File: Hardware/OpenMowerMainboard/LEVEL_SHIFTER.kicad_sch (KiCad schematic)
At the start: 3 parts, among them Q16 BSS138

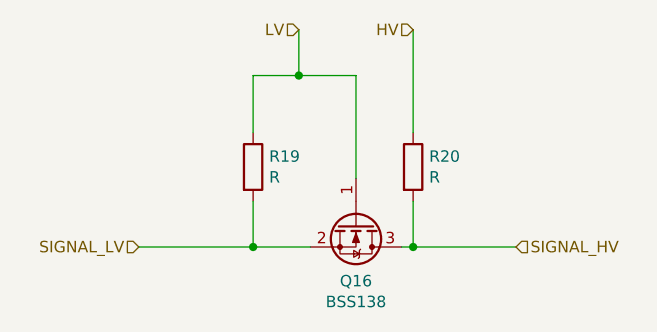
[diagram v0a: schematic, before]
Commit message: minor changes
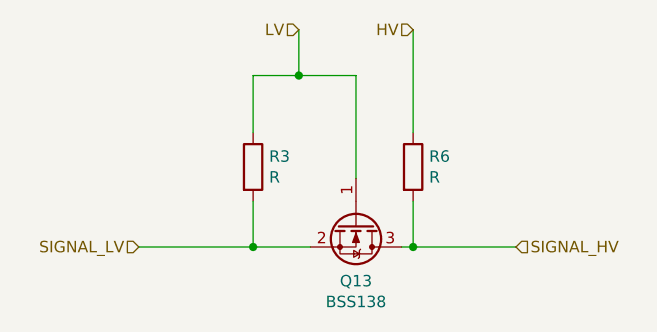
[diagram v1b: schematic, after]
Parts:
- renumbered Q16 to Q13, R19 to R3, R20 to R6
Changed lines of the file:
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@@
   (symbol (lib_id "Transistor_FET:BSS138") (at 114.3 76.2 270)
     (in_bom yes) (on_board yes)
-    (property "Reference" "Q16" (id 0) (at 114.3 82.5246 90))
+    (property "Reference" "Q13" (id 0) (at 114.3 82.5246 90))
     (property "Value" "BSS138" (id 1) (at 114.3 84.836 90))
     (property "Footprint" "Package_TO_SOT_SMD:SOT-23" (id 2) (at 112.395 81.28 0)
@@
   (symbol (lib_id "Device:R") (at 102.87 69.85 0)
     (in_bom yes) (on_board yes)
-    (property "Reference" "R19" (id 0) (at 104.648 68.6816 0)
+    (property "Reference" "R3" (id 0) (at 104.648 68.6816 0)
       (effects (font (size 1.27 1.27)) (justify left))
     )
@@
   (symbol (lib_id "Device:R") (at 120.65 69.85 0)
     (in_bom yes) (on_board yes)
-    (property "Reference" "R20" (id 0) (at 122.428 68.6816 0)
+    (property "Reference" "R6" (id 0) (at 122.428 68.6816 0)
       (effects (font (size 1.27 1.27)) (justify left))
     )

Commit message: minor changes
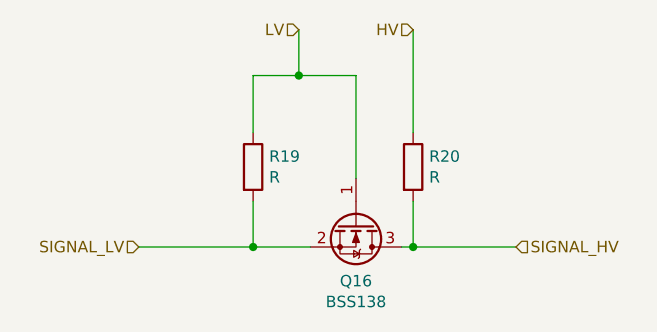
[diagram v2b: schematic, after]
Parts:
- renumbered Q13 to Q16, R3 to R19, R6 to R20
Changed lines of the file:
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@@
   (symbol (lib_id "Transistor_FET:BSS138") (at 114.3 76.2 270)
     (in_bom yes) (on_board yes)
-    (property "Reference" "Q13" (id 0) (at 114.3 82.5246 90))
+    (property "Reference" "Q16" (id 0) (at 114.3 82.5246 90))
     (property "Value" "BSS138" (id 1) (at 114.3 84.836 90))
     (property "Footprint" "Package_TO_SOT_SMD:SOT-23" (id 2) (at 112.395 81.28 0)
@@
   (symbol (lib_id "Device:R") (at 102.87 69.85 0)
     (in_bom yes) (on_board yes)
-    (property "Reference" "R3" (id 0) (at 104.648 68.6816 0)
+    (property "Reference" "R19" (id 0) (at 104.648 68.6816 0)
       (effects (font (size 1.27 1.27)) (justify left))
     )
@@
   (symbol (lib_id "Device:R") (at 120.65 69.85 0)
     (in_bom yes) (on_board yes)
-    (property "Reference" "R6" (id 0) (at 122.428 68.6816 0)
+    (property "Reference" "R20" (id 0) (at 122.428 68.6816 0)
       (effects (font (size 1.27 1.27)) (justify left))
     )
